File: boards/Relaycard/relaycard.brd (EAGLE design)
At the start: 114.3 x 94 mm, 55 parts, among them IC1 ULN2801A, K1 NA, K2 NA, K3 NA, K4 NA, K5 NA, K6 NA, K7 NA, K8 NA, X1 112404, X10 112404, X11 112404, X12 112404, X13 112404, X14 112404, X15 112404, X16 112404, X2 112404, X3 112404, X4 112404, X5 112404, X6 112404, X7 112404, X8 112404, X9 112404

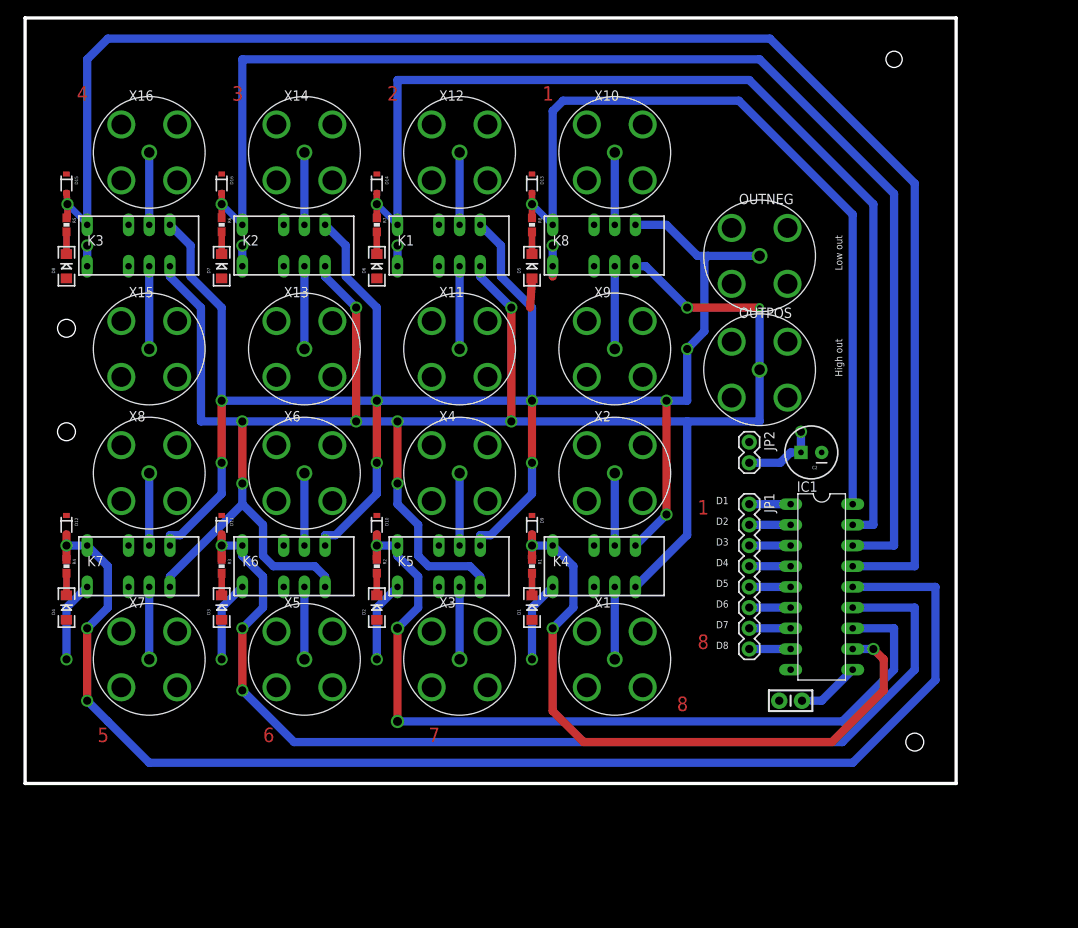
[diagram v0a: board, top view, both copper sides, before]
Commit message: Board update
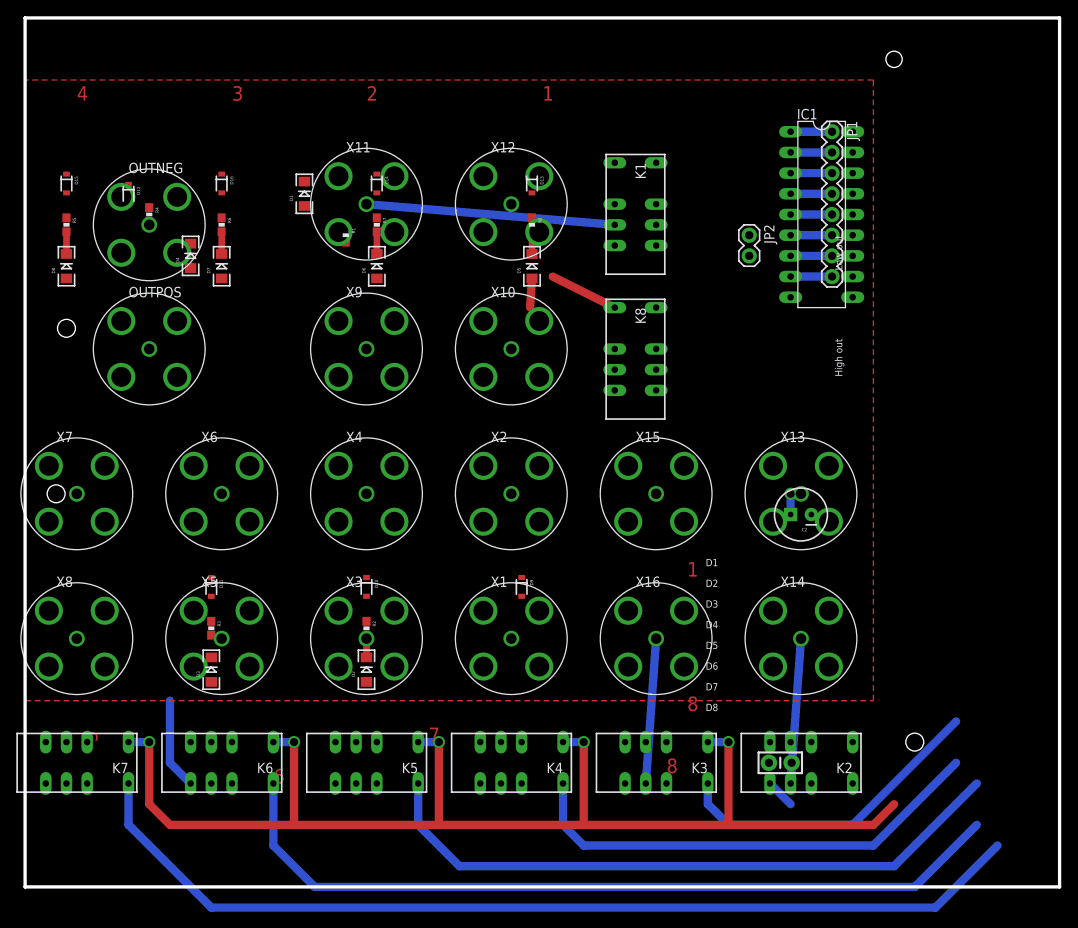
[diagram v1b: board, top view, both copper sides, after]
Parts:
- moved K3 89.8 mm to (74.9, 2.54), turned to 180 degrees
- moved K2 88.9 mm to (92.7, 2.54), turned to 180 degrees
- moved X16 86.2 mm to (74.9, 17.8)
- moved X14 85.3 mm to (92.7, 17.8)
- moved OUTNEG 75.0 mm to (12.7, 68.6)
- moved OUTPOS 75.0 mm to (12.7, 53.3)
- moved X15 64.7 mm to (74.9, 35.6)
- moved X13 63.5 mm to (92.7, 35.6)
- moved D1 58.0 mm to (31.8, 72.4)
- moved JP1 46.8 mm to (96.5, 80.0)
- moved R1 46.6 mm to (36.8, 67.3)
- moved D4 45.8 mm to (17.8, 64.8)
- moved IC1 45.7 mm to (95.2, 69.8)
- moved R4 44.4 mm to (12.7, 69.8)
- moved D12 41.3 mm to (10.2, 72.4)
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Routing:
- net OUTPOS: track 253.6 -> 0.00 mm, vias 10 -> 0
- net OUTNEG: track 248.3 -> 14.8 mm, vias 9 -> 0
- net RELAY3: track 162.1 -> 0.00 mm, vias 1 -> 0
- net RELAY4: track 191.7 -> 39.3 mm, vias 1 -> 0
- net RELAY2: track 131.1 -> 0.00 mm, vias 1 -> 0
- net RELAY1: track 99.3 -> 0.00 mm, vias 1 -> 0
- net VCC: track 70.9 -> 169.2 mm, vias 9 -> 6
- net RELAY5: track 159.9 -> 119.1 mm, vias 3 -> 0
- net RELAY6: track 129.6 -> 99.2 mm, vias 3 -> 0
- net RELAY7: track 103.1 -> 80.0 mm, vias 3 -> 0
- net RELAY8: track 81.0 -> 58.6 mm, vias 3 -> 0
- net N$31: track 10.2 -> 30.6 mm
- net R4: track 10.2 -> 0.00 mm
- net N$35: track 10.2 -> 0.00 mm
- net N$33: track 10.2 -> 0.00 mm
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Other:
- board size 114.3 x 94 mm -> 127 x 106.7 mm
